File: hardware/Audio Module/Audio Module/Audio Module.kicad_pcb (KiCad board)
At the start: 2 copper layers, 21.5 x 33.1 mm, 20 parts, among them IC1 SGTL5000XNLA3R2, IC2 AP7313-18SRG-7, J1 Conn_02x08

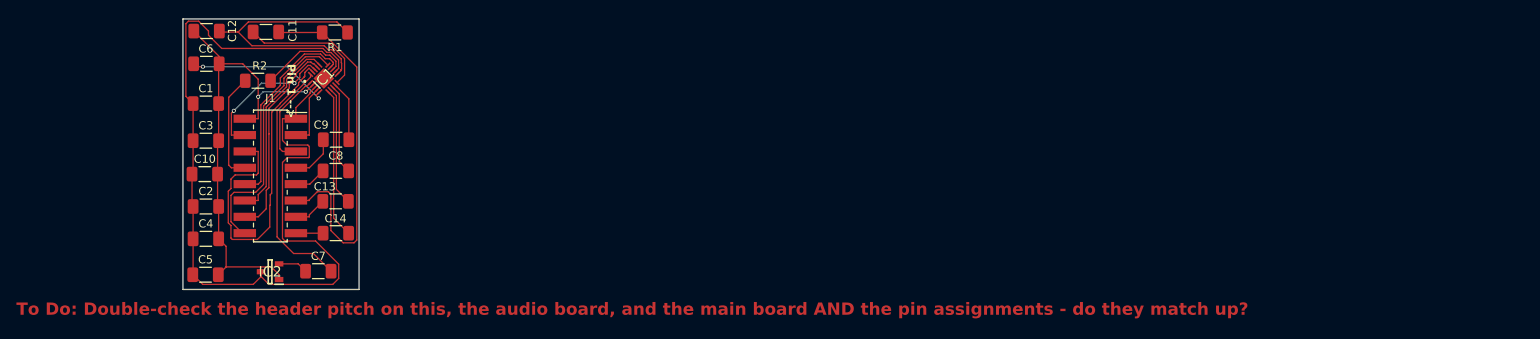
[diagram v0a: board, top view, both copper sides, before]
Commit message: Working on v2 of HW
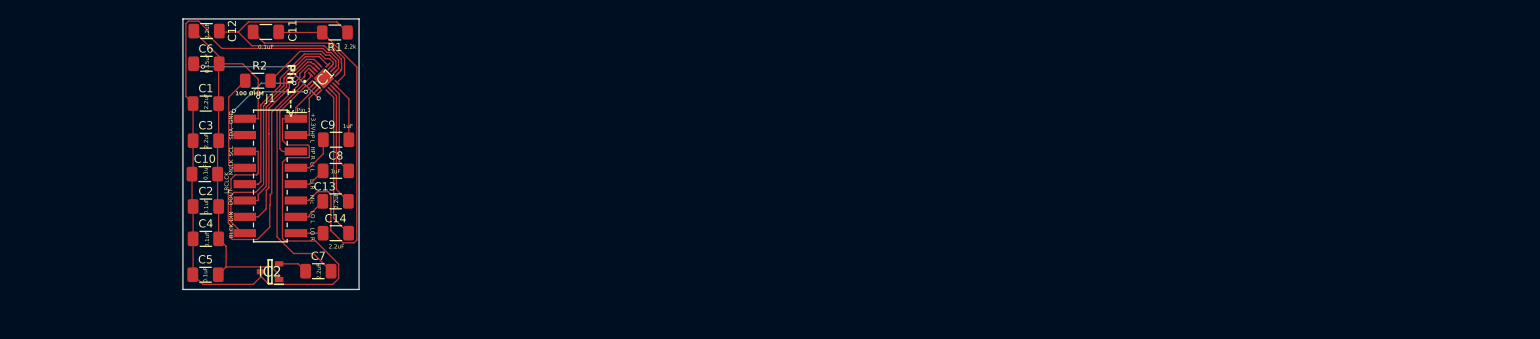
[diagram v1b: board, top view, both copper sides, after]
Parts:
- R2: value 100 -> 100 OHM
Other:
- board text added: "+3.3V"
- board text added: "BLCK"
- board text added: "DIN"
- board text added: "DOUT"
- board text added: "GND"
- board text added: "HP L"
- board text added: "HP R"
- board text added: "LI L"
- board text added: "LI R"
- board text added: "LO L"
- board text added: "LO R"
- board text added: "LRCLCK"
- board text added: "MCLK"
- board text added: "Mic"
- board text added: "Pin 1"
- board text added: "SCL"
- board text added: "SDA"
- board text removed: "To Do: Double-check the header pitch on this, the audio board, and the main board AND the pin assignments - do they match up?"
